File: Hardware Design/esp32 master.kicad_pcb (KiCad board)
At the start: 2 copper layers, 82.7 x 53.2 mm, 30 parts, among them J1 Barrel_Jack_PTH, J2 Conn_01x06_Socket, J3 Conn_01x05_Socket, J4 Conn_01x02_Socket, J5 Conn_01x04_Socket, J6 Conn_01x04_Socket, U1 LM2596S-5, U2 ESP32-DevKitC

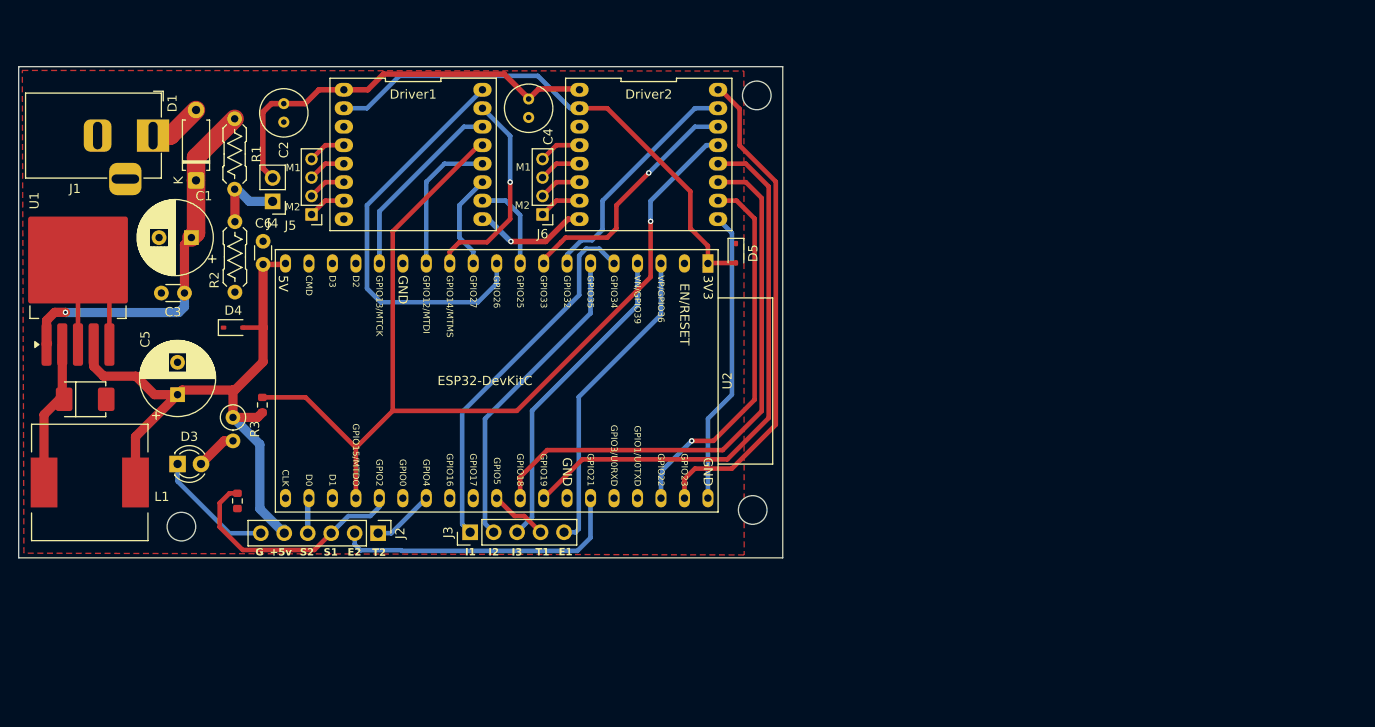
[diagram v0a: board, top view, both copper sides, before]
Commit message: Refactor code structure for improved readability and maintainability
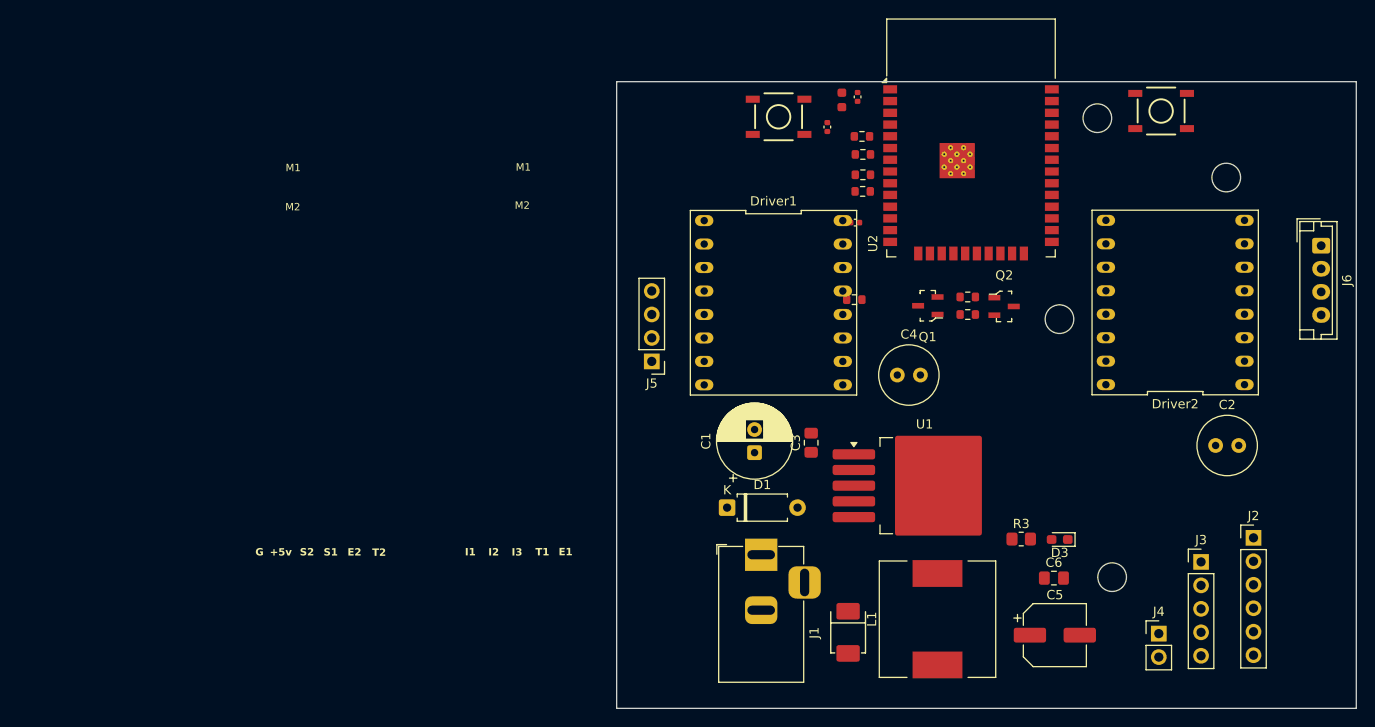
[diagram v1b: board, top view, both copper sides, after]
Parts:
- removed D4, D5: SD36_SOD323, Diode_SMD:D_SOD-323
- added C11: 10uF, PCM_JLCPCB:C_0603, F.Cu at (158.9, 65.6)
- added C7: 0.1uF, SparkFun-Capacitor:C_0402_1005Metric, F.Cu at (160.3, 78.9)
- added C8: 0.1uF, SparkFun-Capacitor:C_0402_1005Metric, F.Cu at (160.6, 65.3)
- added C9: 0.1uF, SparkFun-Capacitor:C_0402_1005Metric, F.Cu at (157.3, 68.5)
- added Q1: BC817-25-TP, digikey-footprints:SOT-23-3, F.Cu at (168.2, 87.9)
- added Q2: BC817-25-TP, digikey-footprints:SOT-23-3, F.Cu at (176.4, 88.0)
- added R6: 10k, SparkFun-Resistor:R_0603_1608Metric, F.Cu at (172.5, 86.9)
- added R7: 0, SparkFun-Resistor:R_0603_1608Metric, F.Cu at (161.2, 75.5)
- added R8: 0, SparkFun-Resistor:R_0603_1608Metric, F.Cu at (160.2, 87.2)
- added ST4: Standoff, SparkFun-Hardware:Standoff, F.Cu at (188.2, 117.2)
- added SW1: SMD_5.2x5.2mm_h1.9mm, SparkFun-Switch:Push_SMD_5.2x5.2mm_h1.9mm, F.Cu at (152.1, 67.4)
- added SW2: SMD_5.2x5.2mm_h1.9mm, SparkFun-Switch:Push_SMD_5.2x5.2mm_h1.9mm, F.Cu at (193.4, 66.8)
- C1: footprint PCM_Capacitor_THT_AKL:CP_Radial_D8.0mm_P3.50mm -> Capacitor_THT:CP_Radial_D8.0mm_P2.50mm
- C2, C4: footprint Capacitor_THT:C_Radial_D5.0mm_H5.0mm_P2.00mm -> Capacitor_THT:C_Radial_D6.3mm_H7.0mm_P2.50mm
- C3, C6: footprint Capacitor_THT:C_Disc_D3.0mm_W1.6mm_P2.50mm -> Capacitor_SMD:C_0805_2012Metric_Pad1.18x1.45mm_HandSolder
- C5: footprint PCM_Capacitor_THT_AKL:CP_Radial_D8.0mm_P3.50mm -> Capacitor_SMD:CP_Elec_6.3x5.4_Nichicon
- D3: footprint LED_THT:LED_D3.0mm -> LED_SMD:LED_0603_1608Metric_Pad1.05x0.95mm_HandSolder
- Driver1, Driver2: footprint tb6612fng:tb6612fng breakout board -> tb6612fng:DIP-16_591_ELL
- J5: footprint Connector_PinHeader_2.00mm:PinHeader_1x04_P2.00mm_Vertical -> Connector_PinHeader_2.54mm:PinHeader_1x04_P2.54mm_Vertical
- J6: footprint Connector_PinHeader_2.00mm:PinHeader_1x04_P2.00mm_Vertical -> Connector_JST:JST_EH_B4B-EH-A_1x04_P2.50mm_Vertical
- R1: value 4.7k -> 10k; footprint PCM_Resistor_THT_US_AKL:R_Axial_DIN0207_L6.3mm_D2.5mm_P7.62mm_Horizontal -> SparkFun-Resistor:R_0603_1608Metric
- R2: footprint PCM_Resistor_THT_US_AKL:R_Axial_DIN0207_L6.3mm_D2.5mm_P7.62mm_Horizontal -> SparkFun-Resistor:R_0603_1608Metric
- R3: footprint Resistor_THT:R_Axial_DIN0207_L6.3mm_D2.5mm_P2.54mm_Vertical -> Resistor_SMD:R_0805_2012Metric_Pad1.20x1.40mm_HandSolder
- U2: value ESP32-DevKitC -> ESP32-WROOM-32D; footprint PCM_Espressif:ESP32-DevKitC -> RF_Module:ESP32-WROOM-32D
- moved ST1 108.5 mm to (186.6, 67.6)
- moved C2 107.4 mm to (199.3, 103.0), turned to 0 degrees
- moved J4 106.7 mm to (193.2, 123.4), turned to 0 degrees
- moved C5 98.5 mm to (181.9, 123.5), turned to 0 degrees
- moved D3 95.8 mm to (182.5, 113.2), turned to 180 degrees
- moved J2 94.7 mm to (203.4, 113.0), turned to 0 degrees
- moved U1 94.4 mm to (167.8, 107.3), turned to 0 degrees
- moved L1 92.9 mm to (169.2, 121.8), turned to 90 degrees
- moved C6 92.1 mm to (181.8, 117.3), turned to 0 degrees
- moved D2 86.3 mm to (159.6, 123.2), turned to -90 degrees
- moved R3 86.3 mm to (178.3, 113.1), turned to 0 degrees
- moved J6 84.3 mm to (210.8, 81.4), turned to -90 degrees
- moved R2 79.9 mm to (172.5, 88.8), turned to 0 degrees
- moved J1 79.9 mm to (150.2, 114.8), turned to 90 degrees
- moved J3 79.2 mm to (197.8, 115.6), turned to 0 degrees
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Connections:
- Driver1 pad 10: /AIN2 -> /MOTOR1_AIN2
- Driver1 pad 11: /AIN1 -> /MOTOR1_AIN1
- Driver1 pad 12: /STBY -> /STBY_PIN
- Driver1 pad 13: /BIN1 -> /MOTOR1_BIN1
- Driver1 pad 14: /BIN2 -> /MOTOR1_BIN2
- Driver1 pad 15: /PWMB -> /MOTOR1_PWMB 
- Driver1 pad 9: /PWMA -> /MOTOR1_PWMA
- Driver2 pad 10: /AIN22 -> /MOTOR2_AIN2
- Driver2 pad 11: /AIN12 -> /MOTOR2_AIN1
- Driver2 pad 12: /STBY -> /STBY_PIN
- Driver2 pad 13: /BIN12 -> /MOTOR2_BIN1
- Driver2 pad 14: /BIN22 -> /MOTOR2_BIN2
- Driver2 pad 15: /PWMB2 -> /MOTOR2_PWMB
- Driver2 pad 9: /PWMA2 -> /MOTOR2_PWMA
- J4 pad 1: Net-(J4-Pin_1) -> /VM
- R1 pad 1: /VM -> /EN
- R1 pad 2: Net-(J4-Pin_1) -> /3v3
- R2 pad 1: Net-(J4-Pin_1) -> Net-(Q1-B)
- R2 pad 2: GND -> /DTR
- R5 pad 1: /STBY -> /STBY_PIN
- U2 pad 1: /3v3 -> GND
- U2 pad 10: /PWMA -> /IO25
- U2 pad 11: /BIN2 -> /IO26
- U2 pad 12: /AIN2 -> /IO27
- U2 pad 13: /BIN1 -> /IO14
- U2 pad 14: GND -> /IO12
- U2 pad 15: /AIN1 -> GND
- U2 pad 16: unconnected-(U2-SD_DATA2/GPIO9-Pad16) -> /IO13
- U2 pad 19: 5V -> unconnected-(U2-SCS/CMD-Pad19)
- U2 pad 2: unconnected-(U2-CHIP_PU-Pad2) -> /3v3
- U2 pad 21: /Servo2 -> unconnected-(U2-SDO/SD0-Pad21)
- U2 pad 23: /STBY -> /IO15
- U2 pad 24: /Servo1 -> /IO2
- U2 pad 25: unconnected-(U2-GPIO0/BOOT/ADC2_CH1-Pad25) -> /IO0
- U2 pad 26: /TRIG2 -> /IO4
- U2 pad 27: unconnected-(U2-GPIO16-Pad27) -> /IO16
- U2 pad 28: unconnected-(U2-GPIO17-Pad28) -> /IO17
- U2 pad 29: /TRIG1 -> /IO5
- U2 pad 3: /ECHO1 -> /EN
- U2 pad 30: /BIN22 -> /IO18
- U2 pad 31: /BIN12 -> /IO19
- U2 pad 32: GND -> unconnected-(U2-NC-Pad32)
- U2 pad 33: /ECHO2 -> /IO21
- U2 pad 34: unconnected-(U2-U0RXD/GPIO3-Pad34) -> /RX
- U2 pad 35: unconnected-(U2-U0TXD/GPIO1-Pad35) -> /TX
- U2 pad 36: /PWMB2 -> /IO22
- U2 pad 37: /PWMA2 -> /IO23
- U2 pad 4: /IR3 -> /SENSOR_VP
- U2 pad 5: /IR1 -> /SENSOR_VN
- U2 pad 6: /IR2 -> /IO34
- U2 pad 7: /AIN22 -> /IO35
- U2 pad 8: /AIN12 -> /IO32
- U2 pad 9: /PWMB -> /IO33
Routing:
- net /STBY: track 108.4 -> 0.00 mm, vias 1 -> 0
- net GND: track 73.4 -> 0.00 mm, vias 1 -> 0
- net 5V: track 71.4 -> 0.00 mm
- net /BIN22: track 59.9 -> 0.00 mm
- net /BIN12: track 59.5 -> 0.00 mm
- net /3v3: track 55.9 -> 0.00 mm
- net /PWMA2: track 53.4 -> 0.00 mm
- net Net-(Driver1-VM): track 45.2 -> 0.00 mm
- net /PWMA: track 44.3 -> 0.00 mm
- net /VM: track 41.4 -> 0.00 mm, vias 1 -> 0
- net /PWMB2: track 40.6 -> 0.00 mm, vias 1 -> 0
- net /IR1: track 40.3 -> 0.00 mm
- net /IR3: track 34.5 -> 0.00 mm
- net /IR2: track 34.2 -> 0.00 mm
- net /ECHO1: track 34.2 -> 0.00 mm
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- added copper zone on In2.Cu, net 5V
- added copper zone on In1.Cu, net GND
- removed copper zone on F.Cu, net GND
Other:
- board size 82.7 x 53.2 mm -> 80 x 67.8 mm
- copper layers 2 -> 4
- board text removed: "Car Model V2"
- board text removed: "S1 GPIO2 S2 GPIO7 IR1 GPIO34 IR2 GPIO35 IR3 GPIO39"
- board text removed: "Ultrasonic 1 Echo1 GPIO36 Trig1 GPIO5 Ultrasonic 2 Echo2 GPIO21 Trig2 GPIO2"
